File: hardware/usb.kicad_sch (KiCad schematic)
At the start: 6 parts, among them J601 USB_C_Receptacle_USB2.0, U601 SRV05-4

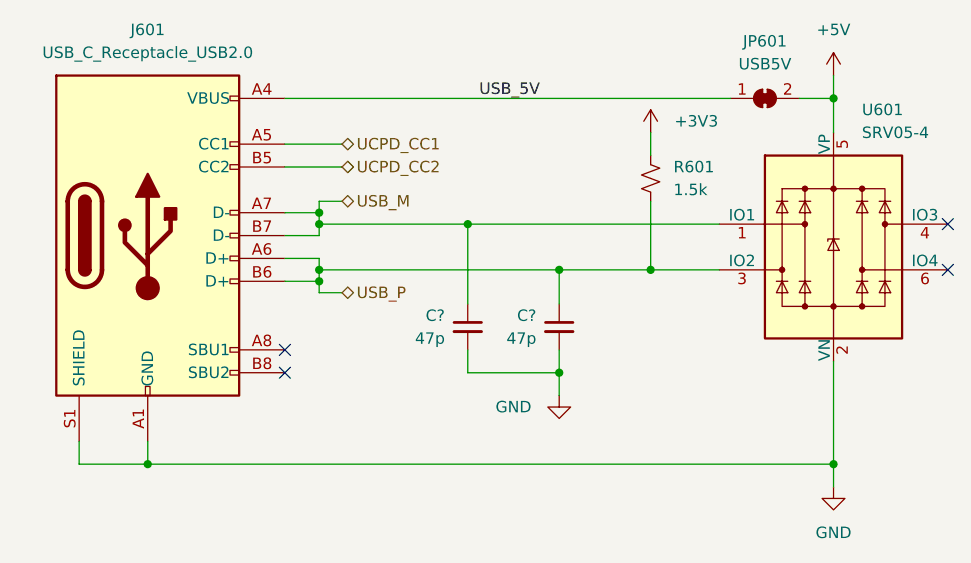
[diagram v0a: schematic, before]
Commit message: work on layout
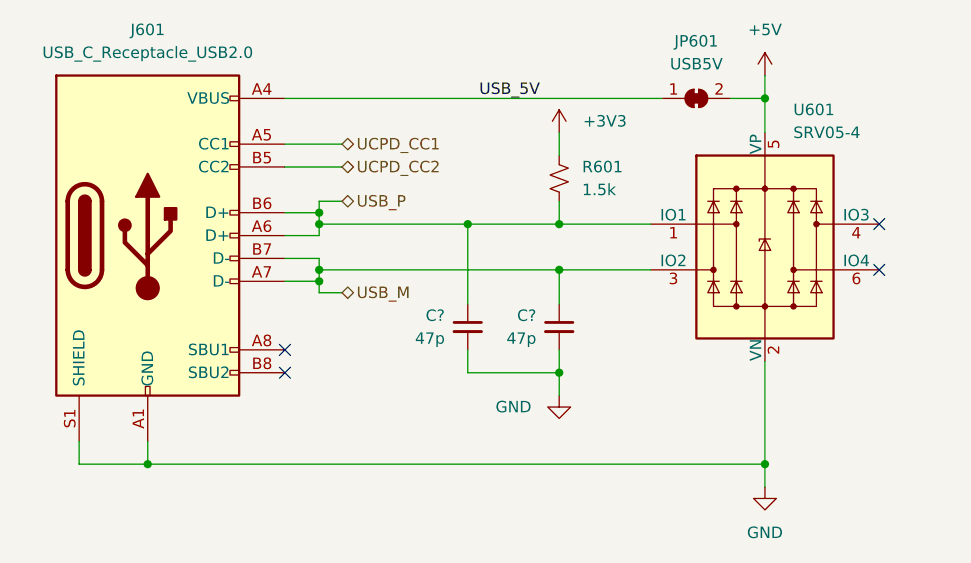
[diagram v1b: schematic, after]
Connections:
- net USB_M: now also C?.1, U601.3 (IO2); no longer C?.1, U601.1 (IO1)
- net USB_P: now also C?.1, U601.1 (IO1); no longer C?.1, U601.3 (IO2)
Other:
- moved on the sheet: JP601, R601, U601
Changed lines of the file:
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@@
     (company "matei repair lab")
   )
-  (junction (at 170.18 93.98) (diameter 0) (color 0 0 0 0)
-  )
-  (junction (at 190.5 74.93) (diameter 0) (color 0 0 0 0)
+  (junction (at 160.02 88.9) (diameter 0) (color 0 0 0 0)
+  )
+  (junction (at 182.88 74.93) (diameter 0) (color 0 0 0 0)
   )
   (junction (at 149.86 88.9) (diameter 0) (color 0 0 0 0)
@@
   (junction (at 133.35 88.9) (diameter 0) (color 0 0 0 0)
   )
-  (junction (at 190.5 115.57) (diameter 0) (color 0 0 0 0)
+  (junction (at 182.88 115.57) (diameter 0) (color 0 0 0 0)
   )
   (junction (at 133.35 87.63) (diameter 0) (color 0 0 0 0)
@@
   (junction (at 133.35 93.98) (diameter 0) (color 0 0 0 0)
   )
-  (no_connect (at 203.2 93.98))
+  (no_connect (at 195.58 93.98))
   (no_connect (at 129.54 105.41))
-  (no_connect (at 203.2 88.9))
+  (no_connect (at 195.58 88.9))
   (no_connect (at 129.54 102.87))
-  (wire (pts (xy 170.18 86.36) (xy 170.18 93.98))
-    (stroke (width 0) (type default))
-  )
-  (wire (pts (xy 190.5 115.57) (xy 190.5 104.14))
+  (wire (pts (xy 182.88 115.57) (xy 182.88 104.14))
+    (stroke (width 0) (type default))
+  )
+  (wire (pts (xy 160.02 86.36) (xy 160.02 88.9))
     (stroke (width 0) (type default))
   )
@@
     (stroke (width 0) (type default))
   )
-  (wire (pts (xy 190.5 74.93) (xy 190.5 78.74))
-    (stroke (width 0) (type default))
-  )
-  (wire (pts (xy 190.5 115.57) (xy 190.5 118.11))
+  (wire (pts (xy 182.88 74.93) (xy 182.88 78.74))
+    (stroke (width 0) (type default))
+  )
+  (wire (pts (xy 182.88 115.57) (xy 182.88 118.11))
     (stroke (width 0) (type default))
   )
@@
     (stroke (width 0) (type default))
   )
-  (wire (pts (xy 190.5 74.93) (xy 190.5 72.39))
-    (stroke (width 0) (type default))
-  )
-  (wire (pts (xy 170.18 93.98) (xy 177.8 93.98))
+  (wire (pts (xy 182.88 74.93) (xy 182.88 72.39))
     (stroke (width 0) (type default))
   )
@@
     (stroke (width 0) (type default))
   )
-  (wire (pts (xy 114.3 115.57) (xy 190.5 115.57))
-    (stroke (width 0) (type default))
-  )
-  (wire (pts (xy 149.86 88.9) (xy 177.8 88.9))
-    (stroke (width 0) (type default))
-  )
-  (wire (pts (xy 129.54 74.93) (xy 179.07 74.93))
-    (stroke (width 0) (type default))
-  )
-  (wire (pts (xy 186.69 74.93) (xy 190.5 74.93))
+  (wire (pts (xy 114.3 115.57) (xy 182.88 115.57))
+    (stroke (width 0) (type default))
+  )
+  (wire (pts (xy 149.86 88.9) (xy 160.02 88.9))
+    (stroke (width 0) (type default))
+  )
+  (wire (pts (xy 129.54 74.93) (xy 171.45 74.93))
+    (stroke (width 0) (type default))
+  )
+  (wire (pts (xy 179.07 74.93) (xy 182.88 74.93))
+    (stroke (width 0) (type default))
+  )
+  (wire (pts (xy 160.02 88.9) (xy 170.18 88.9))
     (stroke (width 0) (type default))
   )
@@
     (stroke (width 0) (type default))
   )
-  (wire (pts (xy 170.18 78.74) (xy 170.18 81.28))
+  (wire (pts (xy 160.02 78.74) (xy 160.02 81.28))
     (stroke (width 0) (type default))
   )
@@
     (effects (font (size 1.27 1.27)) (justify left bottom))
   )
-  (hierarchical_label "USB_M" (shape bidirectional) (at 135.89 86.36 0) (fields_autoplaced)
+  (hierarchical_label "USB_M" (shape bidirectional) (at 135.89 96.52 0) (fields_autoplaced)
     (effects (font (size 1.27 1.27)) (justify left))
   )
@@
     (effects (font (size 1.27 1.27)) (justify left))
   )
-  (hierarchical_label "USB_P" (shape bidirectional) (at 135.89 96.52 0) (fields_autoplaced)
+  (hierarchical_label "USB_P" (shape bidirectional) (at 135.89 86.36 0) (fields_autoplaced)
     (effects (font (size 1.27 1.27)) (justify left))
   )
@@
     )
   )
-  (symbol (lib_id "Jumper:SolderJumper_2_Bridged") (at 182.88 74.93 0) (unit 1)
+  (symbol (lib_id "Jumper:SolderJumper_2_Bridged") (at 175.26 74.93 0) (unit 1)
     (in_bom yes) (on_board yes) (dnp no) (fields_autoplaced)
-    (property "Reference" "JP601" (at 182.88 68.58 0)
-      (effects (font (size 1.27 1.27)))
-    )
-    (property "Value" "USB5V" (at 182.88 71.12 0)
-      (effects (font (size 1.27 1.27)))
-    )
-    (property "Footprint" "Jumper:SolderJumper-2_P1.3mm_Bridged_RoundedPad1.0x1.5mm" (at 182.88 74.93 0)
-      (effects (font (size 1.27 1.27)) hide)
-    )
-    (property "Datasheet" "~" (at 182.88 74.93 0)
+    (property "Reference" "JP601" (at 175.26 68.58 0)
+      (effects (font (size 1.27 1.27)))
+    )
+    (property "Value" "USB5V" (at 175.26 71.12 0)
+      (effects (font (size 1.27 1.27)))
+    )
+    (property "Footprint" "Jumper:SolderJumper-2_P1.3mm_Bridged_RoundedPad1.0x1.5mm" (at 175.26 74.93 0)
+      (effects (font (size 1.27 1.27)) hide)
+    )
+    (property "Datasheet" "~" (at 175.26 74.93 0)
       (effects (font (size 1.27 1.27)) hide)
     )
@@
     )
   )
-  (symbol (lib_id "Power_Protection:SRV05-4") (at 190.5 91.44 0) (unit 1)
-    (in_bom yes) (on_board yes) (dnp no) (fields_autoplaced)
-    (property "Reference" "U601" (at 193.6497 76.2 0)
+  (symbol (lib_id "Power_Protection:SRV05-4") (at 182.88 91.44 0) (unit 1)
+    (in_bom yes) (on_board yes) (dnp no)
+    (property "Reference" "U601" (at 186.0297 76.2 0)
       (effects (font (size 1.27 1.27)) (justify left))
     )
-    (property "Value" "SRV05-4" (at 193.6497 78.74 0)
+    (property "Value" "SRV05-4" (at 186.0297 78.74 0)
       (effects (font (size 1.27 1.27)) (justify left))
     )
-    (property "Footprint" "Package_TO_SOT_SMD:SOT-23-6" (at 208.28 102.87 0)
-      (effects (font (size 1.27 1.27)) hide)
-    )
-    (property "Datasheet" "http://www.onsemi.com/pub/Collateral/SRV05-4-D.PDF" (at 190.5 91.44 0)
+    (property "Footprint" "Package_TO_SOT_SMD:SOT-23-6" (at 200.66 102.87 0)
+      (effects (font (size 1.27 1.27)) hide)
+    )
+    (property "Datasheet" "http://www.onsemi.com/pub/Collateral/SRV05-4-D.PDF" (at 182.88 91.44 0)
       (effects (font (size 1.27 1.27)) hide)
     )
@@
     )
   )
-  (symbol (lib_id "power:+5V") (at 190.5 72.39 0) (unit 1)
+  (symbol (lib_id "power:+5V") (at 182.88 72.39 0) (unit 1)
     (in_bom yes) (on_board yes) (dnp no) (fields_autoplaced)
-    (property "Reference" "#PWR0603" (at 190.5 76.2 0)
-      (effects (font (size 1.27 1.27)) hide)
-    )
-    (property "Value" "+5V" (at 190.5 67.31 0)
-      (effects (font (size 1.27 1.27)))
-    )
-    (property "Footprint" "" (at 190.5 72.39 0)
-      (effects (font (size 1.27 1.27)) hide)
-    )
-    (property "Datasheet" "" (at 190.5 72.39 0)
+    (property "Reference" "#PWR0603" (at 182.88 76.2 0)
+      (effects (font (size 1.27 1.27)) hide)
+    )
+    (property "Value" "+5V" (at 182.88 67.31 0)
+      (effects (font (size 1.27 1.27)))
+    )
+    (property "Footprint" "" (at 182.88 72.39 0)
+      (effects (font (size 1.27 1.27)) hide)
+    )
+    (property "Datasheet" "" (at 182.88 72.39 0)
       (effects (font (size 1.27 1.27)) hide)
     )
@@
     )
   )
-  (symbol (lib_id "power:+3V3") (at 170.18 78.74 0) (unit 1)
+  (symbol (lib_id "power:+3V3") (at 160.02 78.74 0) (unit 1)
     (in_bom yes) (on_board yes) (dnp no)
-    (property "Reference" "#PWR0601" (at 170.18 82.55 0)
-      (effects (font (size 1.27 1.27)) hide)
-    )
-    (property "Value" "+3V3" (at 175.26 77.47 0)
-      (effects (font (size 1.27 1.27)))
-    )
-    (property "Footprint" "" (at 170.18 78.74 0)
-      (effects (font (size 1.27 1.27)) hide)
-    )
-    (property "Datasheet" "" (at 170.18 78.74 0)
+    (property "Reference" "#PWR0601" (at 160.02 82.55 0)
+      (effects (font (size 1.27 1.27)) hide)
+    )
+    (property "Value" "+3V3" (at 165.1 77.47 0)
+      (effects (font (size 1.27 1.27)))
+    )
+    (property "Footprint" "" (at 160.02 78.74 0)
+      (effects (font (size 1.27 1.27)) hide)
+    )
+    (property "Datasheet" "" (at 160.02 78.74 0)
       (effects (font (size 1.27 1.27)) hide)
     )
@@
     )
   )
-  (symbol (lib_id "Device:R_Small_US") (at 170.18 83.82 0) (unit 1)
+  (symbol (lib_id "Device:R_Small_US") (at 160.02 83.82 0) (unit 1)
     (in_bom yes) (on_board yes) (dnp no) (fields_autoplaced)
-    (property "Reference" "R601" (at 172.72 82.55 0)
+    (property "Reference" "R601" (at 162.56 82.55 0)
       (effects (font (size 1.27 1.27)) (justify left))
     )
-    (property "Value" "1.5k" (at 172.72 85.09 0)
+    (property "Value" "1.5k" (at 162.56 85.09 0)
       (effects (font (size 1.27 1.27)) (justify left))
     )
-    (property "Footprint" "Resistor_SMD:R_0402_1005Metric" (at 170.18 83.82 0)
-      (effects (font (size 1.27 1.27)) hide)
-    )
-    (property "Datasheet" "~" (at 170.18 83.82 0)
+    (property "Footprint" "Resistor_SMD:R_0402_1005Metric" (at 160.02 83.82 0)
+      (effects (font (size 1.27 1.27)) hide)
+    )
+    (property "Datasheet" "~" (at 160.02 83.82 0)
       (effects (font (size 1.27 1.27)) hide)
     )
@@
     )
   )
-  (symbol (lib_id "power:GND") (at 190.5 118.11 0) (unit 1)
+  (symbol (lib_id "power:GND") (at 182.88 118.11 0) (unit 1)
     (in_bom yes) (on_board yes) (dnp no) (fields_autoplaced)
-    (property "Reference" "#PWR0604" (at 190.5 124.46 0)
-      (effects (font (size 1.27 1.27)) hide)
-    )
-    (property "Value" "GND" (at 190.5 123.19 0)
-      (effects (font (size 1.27 1.27)))
-    )
-    (property "Footprint" "" (at 190.5 118.11 0)
-      (effects (font (size 1.27 1.27)) hide)
-    )
-    (property "Datasheet" "" (at 190.5 118.11 0)
-      (effects (font (size 1.27 1.27)) hide)
-    )
+    (property "Reference" "#PWR0604" (at 182.88 124.46 0)
+      (effects (font (size 1.27 1.27)) hide)
+    )
+    (property "Value" "GND" (at 182.88 123.19 0)
+      (effects (font (size 1.27 1.27)))
+    )
+    (property "Footprint" "" (at 182.88 118.11 0)
+      (effects (font (size 1.27 1.27)) hide)
+    )
+    (property "Datasheet" "" (at 182.88 118.11 0)
+      (effects (font (size 1.27 1.27)) hide)
+    )
